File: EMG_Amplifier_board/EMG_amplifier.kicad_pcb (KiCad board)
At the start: 2 copper layers, 50.1 x 39.8 mm, 51 parts, among them J1 Conn_01x04_Socket, J2 Conn_01x04_Pin, J3 Conn_01x06_Pin, J4 Conn_01x06_Socket, J5 Conn_01x04_Pin, J6 Conn_01x01_Pin, U1 LPV821DBVR, U2 INA333xxDGK, U3 LPV821DBVR, U5 LPV821DBVR, U6 LPV821DBVR, U7 TPD2E001DRLR, U8 TLV8542DR

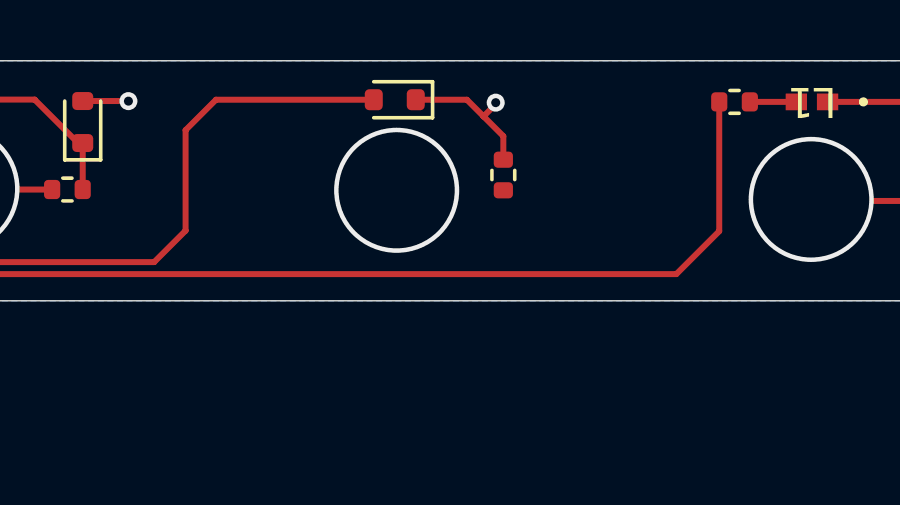
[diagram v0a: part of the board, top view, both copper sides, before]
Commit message: minor link addition
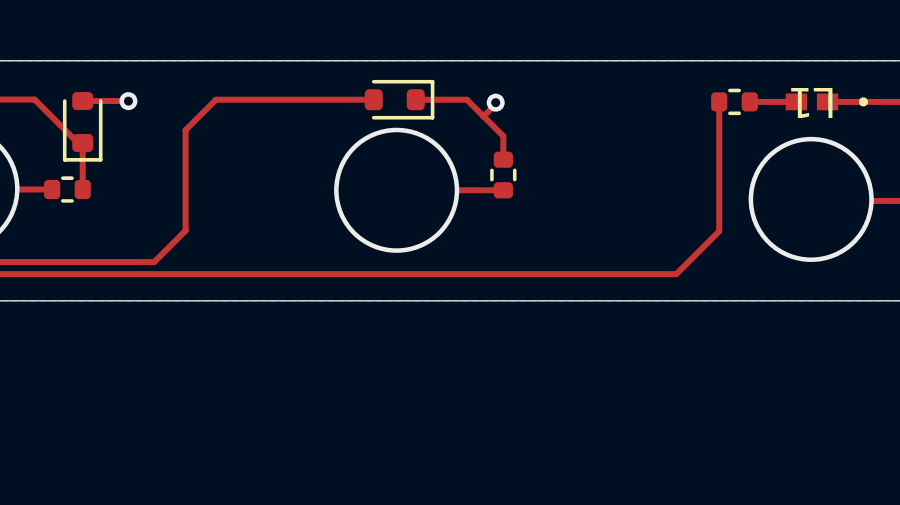
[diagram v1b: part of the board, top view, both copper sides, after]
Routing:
- net input_ER: track 0.00 -> 3.56 mm
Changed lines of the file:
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@@
 		(net 26)
+	)
+	(segment
+		(start 81.8388 86.8172)
+		(end 85.3948 86.8172)
+		(width 0.2)
+		(layer "F.Cu")
+		(net 27)
 	)
 	(via
